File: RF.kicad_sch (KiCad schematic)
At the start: 0 parts

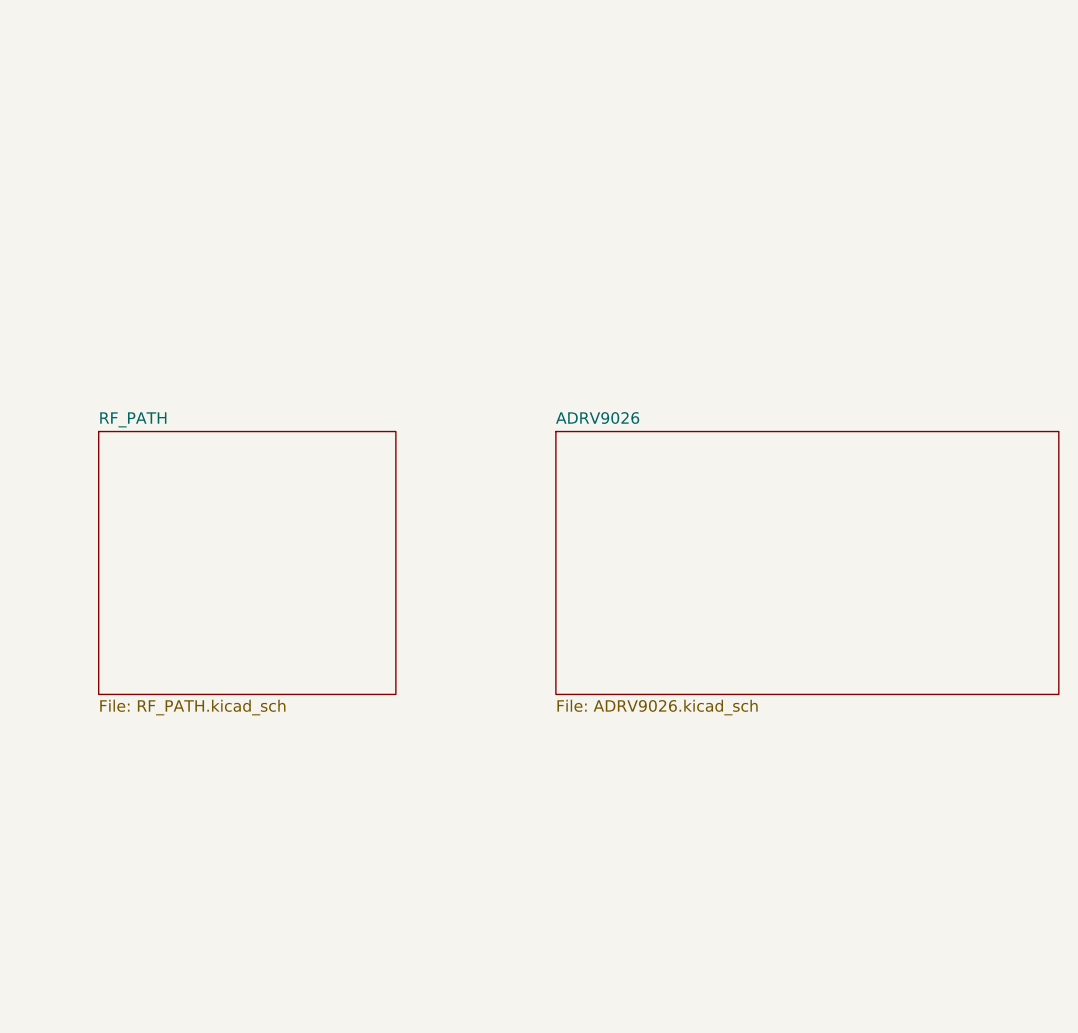
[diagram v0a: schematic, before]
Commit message: pushing the schematics works
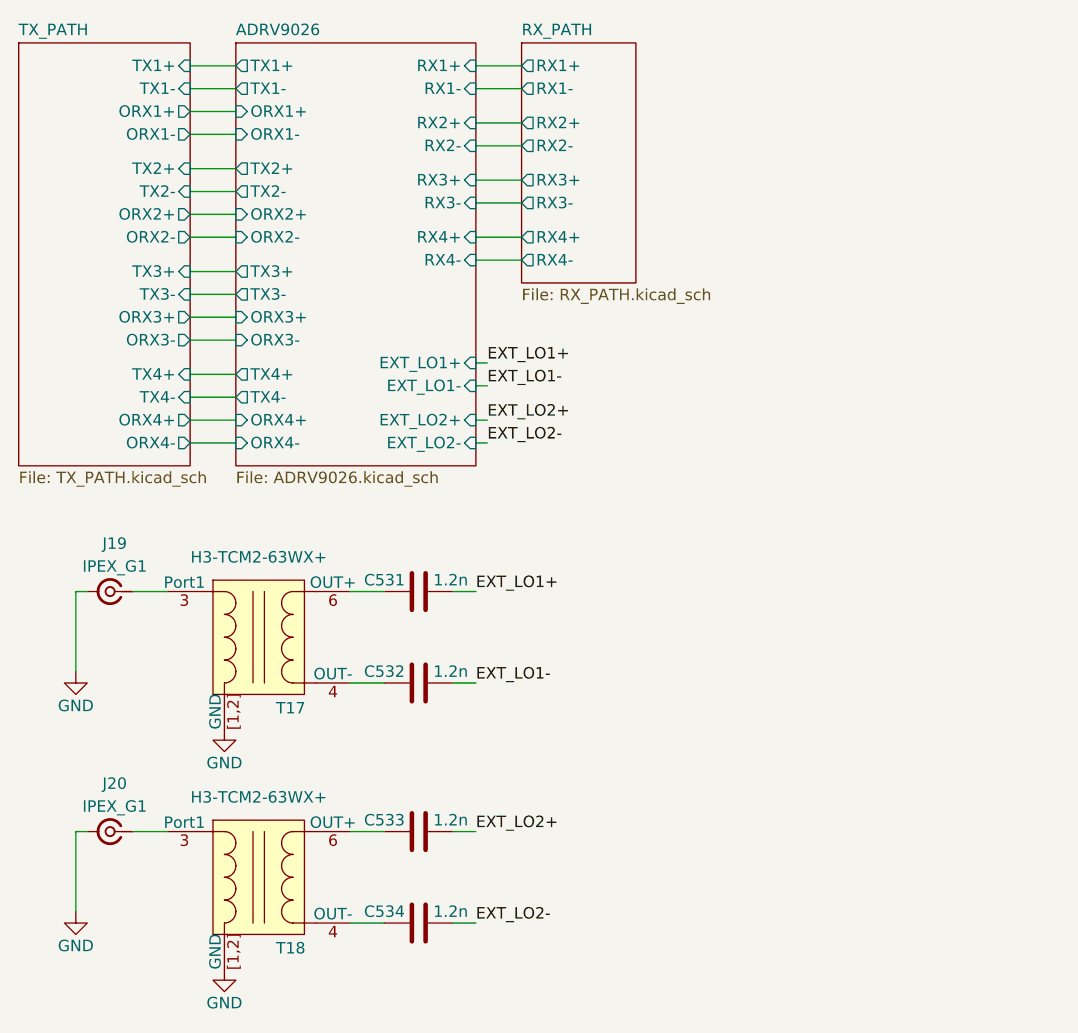
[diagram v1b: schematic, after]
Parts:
- added C531, C532, C533, C534: 1.2n, Capacitor_SMD:C_0201_0603Metric, symbol Device:C
- added J19, J20: IPEX_G1, Connector_Coaxial:U.FL_Hirose_U.FL-R-SMT-1_Vertical, symbol Connector:Conn_Coaxial_Small
- added T17, T18: H3-TCM2-63WX+, dfdtc_RF:HT_TCP_2_25P, symbol dfdtc_RF:H3-TCM2-63WX+
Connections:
- new net: C534.1, T18.4 (OUT-)
- new net: J19.1 (In), T17.3 (Port1)
- new net: C532.1, T17.4 (OUT-)
- new net: C531.1, T17.6 (OUT+)
- new net: C533.1, T18.6 (OUT+)
- new net: J20.1 (In), T18.3 (Port1)
- new net EXT_LO1+: C531.2
- new net EXT_LO1-: C532.2
- new net EXT_LO2+: C533.2
- new net EXT_LO2-: C534.2
- new net GND: J19.2 (Ext), J20.2 (Ext), T17.5 (NC), T17.[1,2] (GND), T18.5 (NC), T18.[1,2] (GND)
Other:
- removed sheet RF_PATH
- added sheet RX_PATH (RX_PATH.kicad_sch)
- added sheet TX_PATH (TX_PATH.kicad_sch)
- sheet ADRV9026 ports: added EXT_LO1+, EXT_LO1-, EXT_LO2+, EXT_LO2-, ORX1+, ORX1-, ORX2+, ORX2-, ORX3+, ORX3-, ORX4+, ORX4-, RX1+, RX1-, RX2+, RX2-, RX3+, RX3-, RX4+, RX4-, TX1+, TX1-, TX2+, TX2-, TX3+, TX3-, TX4+, TX4-; removed none
